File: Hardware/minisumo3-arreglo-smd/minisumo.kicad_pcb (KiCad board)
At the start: 2 copper layers, 17 parts, among them J1 batterly, J2 hc-sr05, J3 sensor, M1 Motor_DC, M2 Motor_DC, SW1 SW_DPST_x2, U1 L293D, U2 L7805

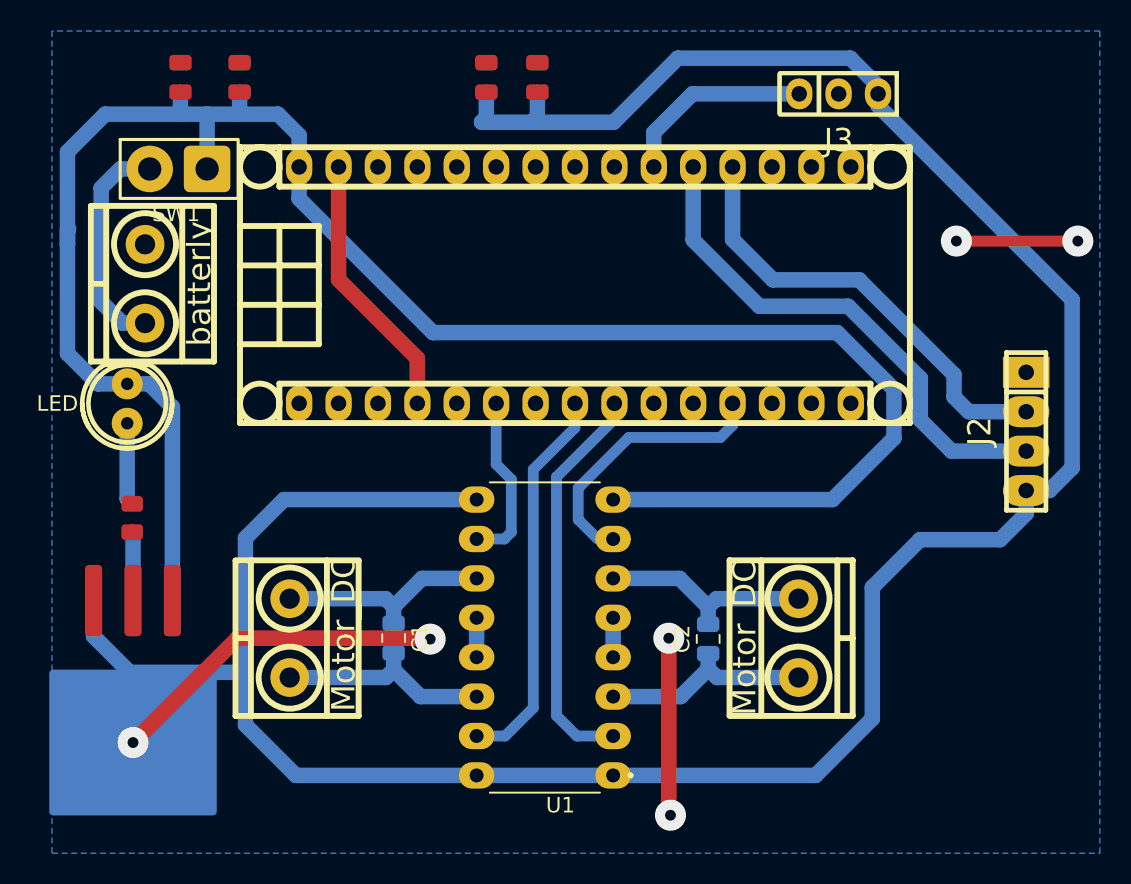
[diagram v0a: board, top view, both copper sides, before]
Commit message: Add files via upload
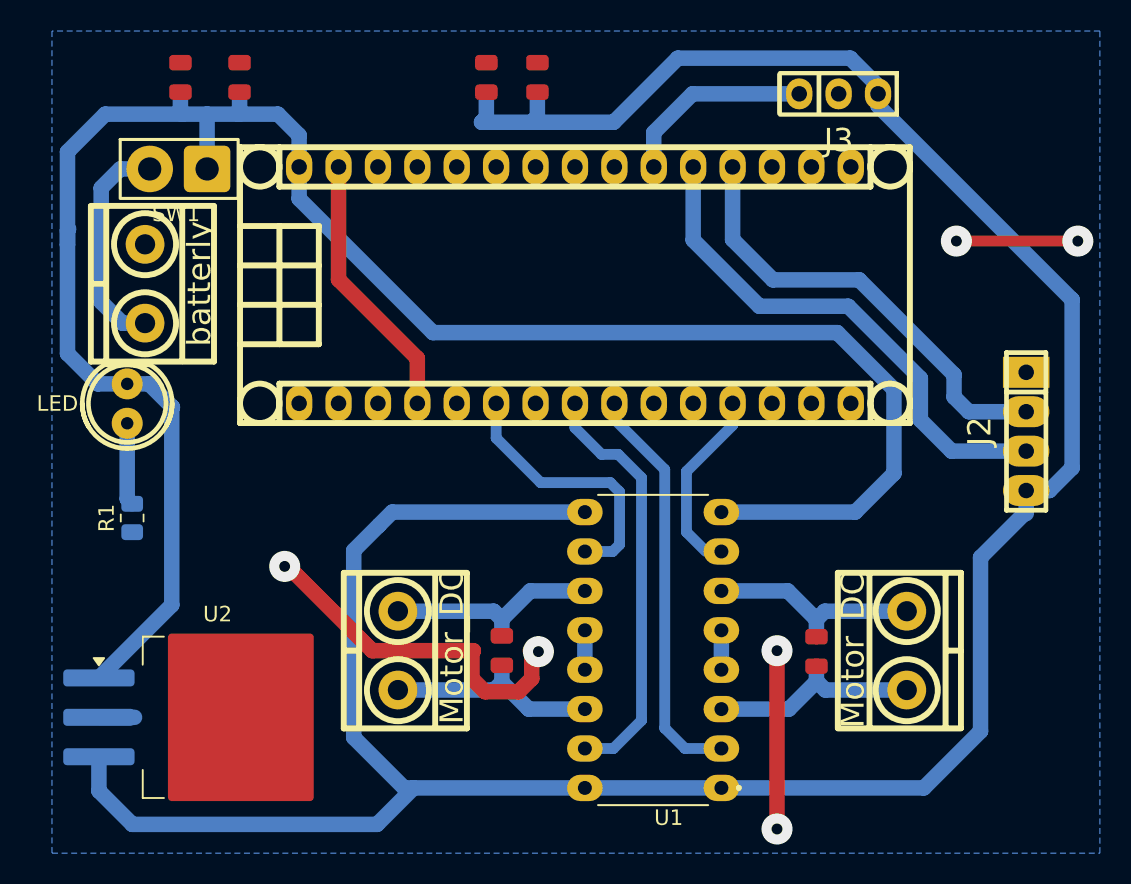
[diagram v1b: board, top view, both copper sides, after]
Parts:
- C1, C2: moved to B.Cu
- R1, U2: moved to F.Cu
- moved M1 7.02 mm to (138.6, 96.7)
- moved M2 7.02 mm to (105.8, 96.7)
- moved C1 7.02 mm to (112.5, 96.7)
- moved U1 7.02 mm to (122.3, 96.6)
- moved C2 7.02 mm to (132.8, 96.7)
- moved U2 5.45 mm to (94.2, 101.0), turned to 0 degrees
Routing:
- net +5V: track 171.4 -> 178.9 mm
- net motor2A: track 11.1 -> 17.5 mm
- net motor1B: track 17.8 -> 12.3 mm
- net motor2B: track 25.5 -> 27.6 mm
- net VCC: track 128.1 -> 129.7 mm
- net GND: track 68.4 -> 67.5 mm
- net motor1A: track 25.9 -> 26.5 mm
